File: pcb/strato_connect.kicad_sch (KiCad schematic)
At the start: 42 parts, among them J1 Conn_Coaxial, J2 Conn_02x03_Odd_Even, J3 Conn_01x04_Pin, J4 Conn_01x02_Pin, J5 Conn_01x05_Pin, SW1 SW_SPST, SW2 SW_SPST, U1 TPS565242, U2 ATmega328PB-A, U4 RF4463F30, Y1 CSTNE16M0V530000R0

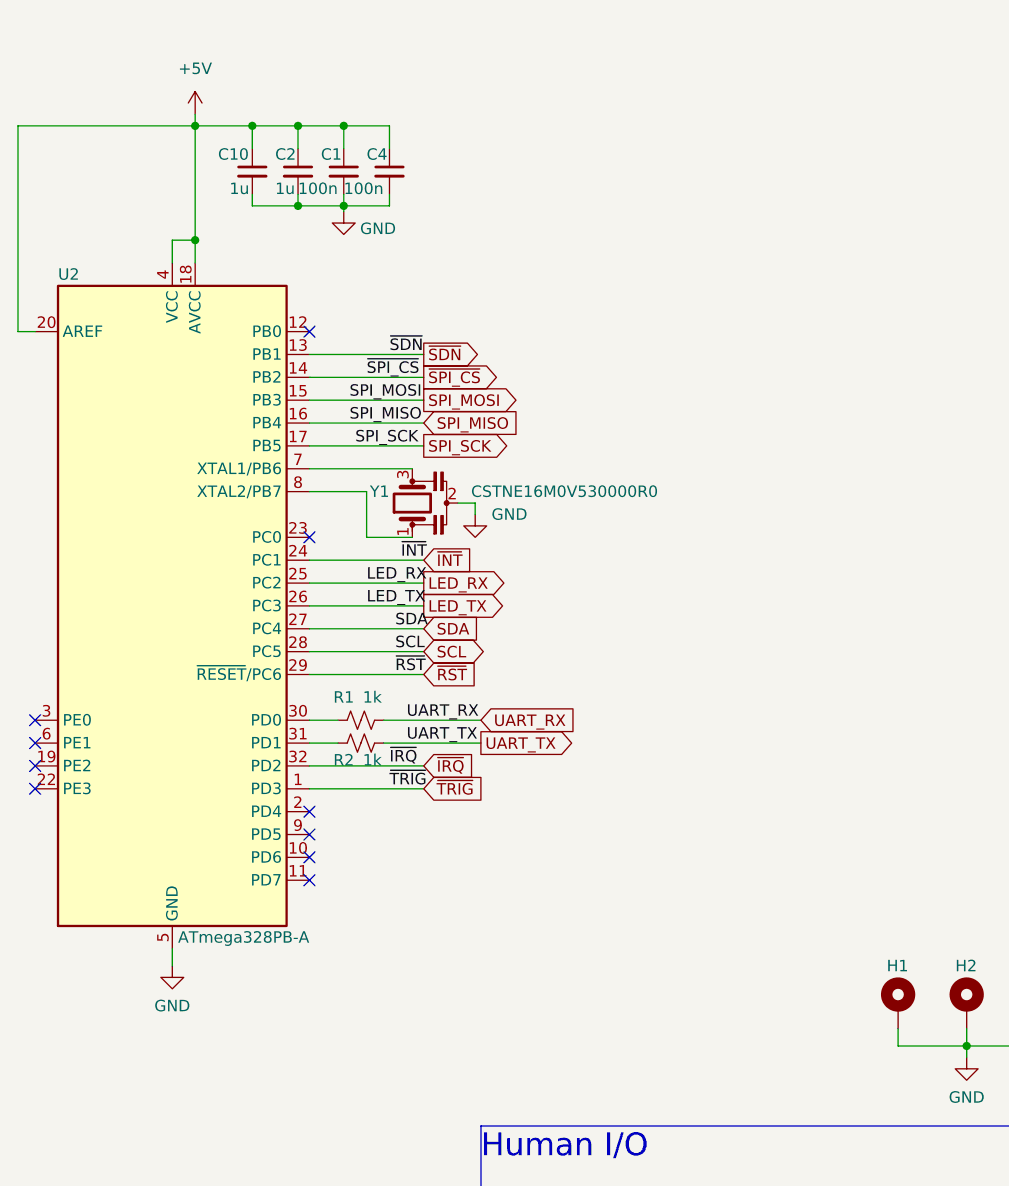
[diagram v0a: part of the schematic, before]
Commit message: rough layout of the rev2 pcb
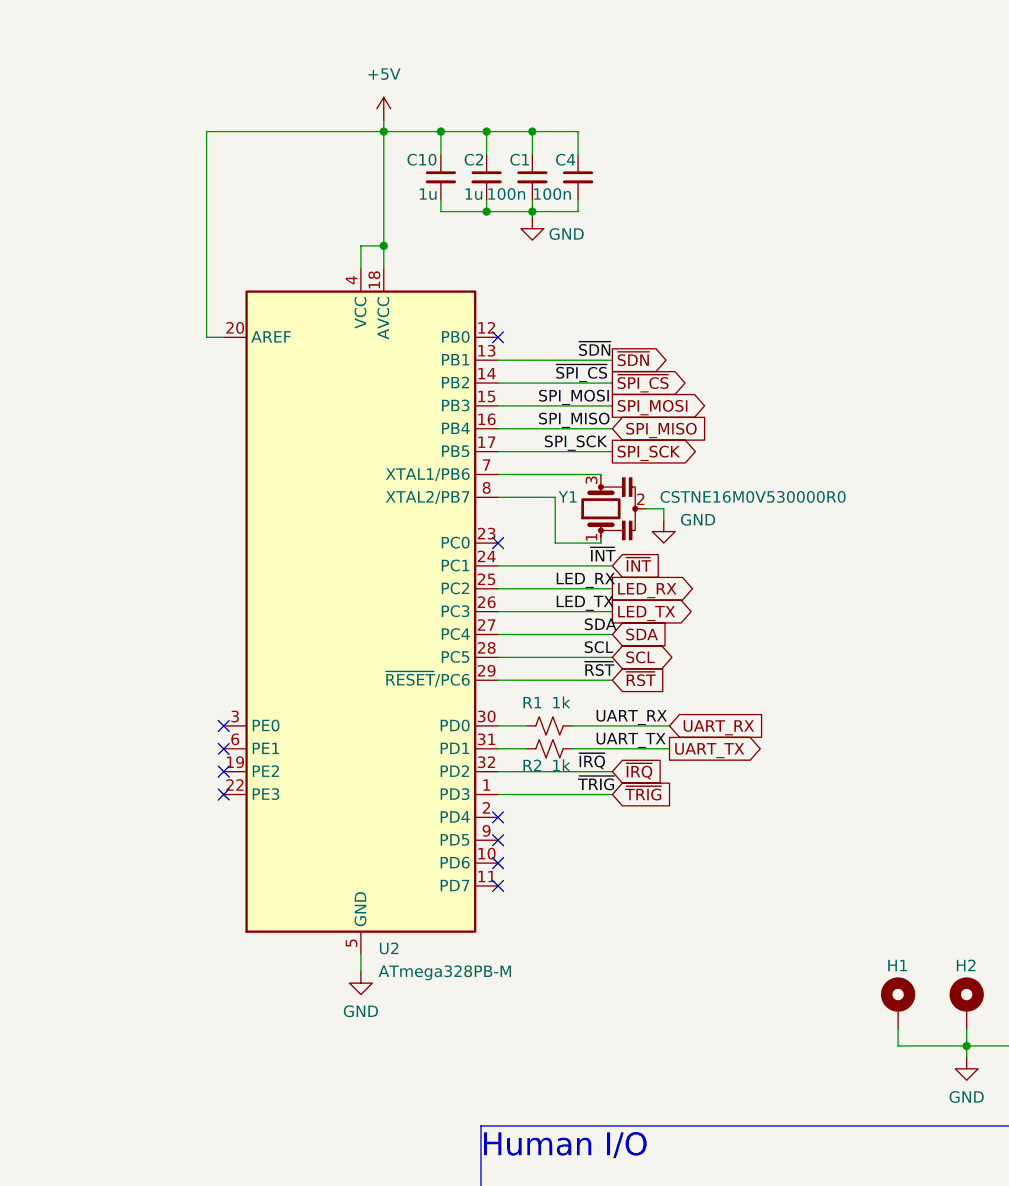
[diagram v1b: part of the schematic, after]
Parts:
- removed U2: ATmega328PB-A, Package_QFP:TQFP-32_7x7mm_P0.8mm, symbol MCU_Microchip_ATmega:ATmega328PB-A
- added U2: ATmega328PB-M, Package_DFN_QFN:QFN-32-1EP_5x5mm_P0.5mm_EP3.1x3.1mm, symbol MCU_Microchip_ATmega:ATmega328PB-M
- C11, C9: footprint Capacitor_SMD:CP_Elec_5x5.3 -> Capacitor_SMD:C_0603_1608Metric
- J2: footprint Connector_PinHeader_2.54mm:PinHeader_2x03_P2.54mm_Vertical -> Connector_PinHeader_2.54mm:PinHeader_2x03_P2.54mm_Vertical_SMD
- J3: footprint (none) -> Connector_JST:JST_SH_SM04B-SRSS-TB_1x04-1MP_P1.00mm_Horizontal
- J4: footprint Connector_JST:JST_SH_BM04B-SRSS-TB_1x04-1MP_P1.00mm_Vertical -> Connector_JST:JST_PH_S2B-PH-SM4-TB_1x02-1MP_P2.00mm_Horizontal
- J5: footprint (none) -> Connector_JST:JST_SH_SM05B-SRSS-TB_1x05-1MP_P1.00mm_Horizontal
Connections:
- net +5V: now also U2.18 (AVCC), U2.20 (AREF), U2.4 (VCC)
- net GND: now also U2.21 (GND), U2.33 (GND), U2.5 (GND)
- net LED_RX: now also U2.25 (PC2)
- net LED_TX: now also U2.26 (PC3)
- net SCL: now also U2.28 (PC5)
- net SDA: now also U2.27 (PC4)
- net SPI_MISO: now also U2.16 (PB4)
- net SPI_MOSI: now also U2.15 (PB3)
- net SPI_SCK: now also U2.17 (PB5)
- net ~{INT}: now also U2.24 (PC1)
- net ~{IRQ}: now also U2.32 (PD2)
- net ~{RST}: now also U2.29 (~{RESET}/PC6)
- net ~{SDN}: now also U2.13 (PB1)
- net ~{SPI_CS}: now also U2.14 (PB2)
- net ~{TRIG}: now also U2.1 (PD3)
- net at R2.1: now also U2.31 (PD1)
- net at Y1.1: now also U2.8 (XTAL2/PB7)
- net at Y1.3: now also U2.7 (XTAL1/PB6)
- net at R1.1: now also U2.30 (PD0)
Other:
- moved on the sheet: C1, C10, C2, C4, R1, R2, Y1
